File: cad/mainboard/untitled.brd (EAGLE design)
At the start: 100 x 80 mm, 12 parts

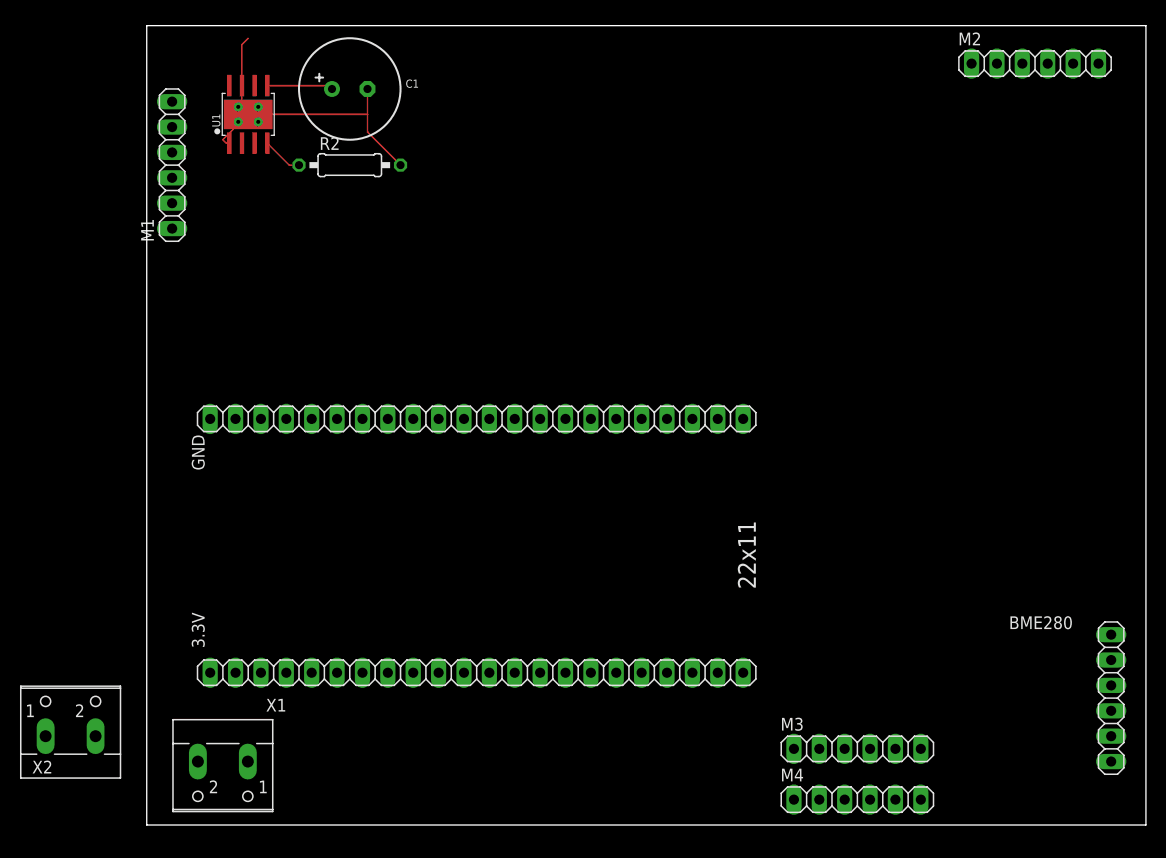
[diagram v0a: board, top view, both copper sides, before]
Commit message: board
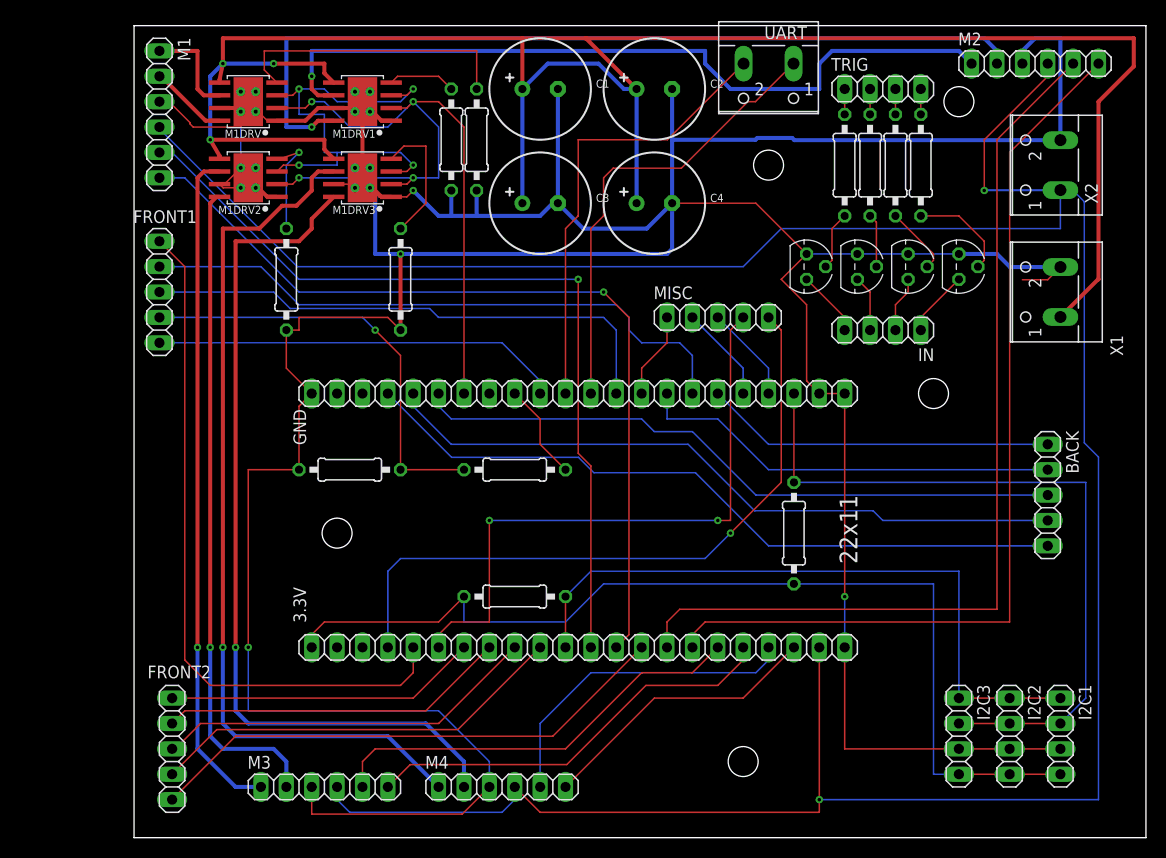
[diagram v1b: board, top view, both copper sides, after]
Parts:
- removed BME280: (no value), pinhead:1X06
- removed U1: (no value), Adafruit DRV8871:MICROBUILDER_HSOP8
- added 1K, 1K1, 1K3, 1K4, 1K5, 1K6, R3: 1k, rcl:0207/10
- added 1K2: 1.8k, rcl:0207/10
- added BACK, FRONT1, FRONT2, MISC: (no value), pinhead:1X05
- added C2, C3, C4: (no value), Adafruit DRV8871:MICROBUILDER_CELEC_3.5MM_10MM
- added I2C1, I2C2, I2C3, IN, TRIG: (no value), pinhead:1X04
- added M1DRV, M1DRV1, M1DRV2, M1DRV3: (no value), Adafruit DRV8871:MICROBUILDER_HSOP8
- added R1, R4, R5: 30k, rcl:0207/10
- added T1, T2, T3, T4: 2N3904, transistor:TO92
- added UART: (no value), con-wago-500:W237-102
- R2: value (none) -> 30k
- moved X2 112.6 mm to (90.2, 66.0), turned to 90 degrees
- moved X1 95.6 mm to (90.2, 53.3), turned to 90 degrees
- moved M3 53.5 mm to (17.8, 3.81)
- moved M4 35.6 mm to (35.6, 3.81)
- moved C1 19.0 mm to (39.4, 73.7)
- moved R2 13.0 mm to (33.0, 68.6), turned to 270 degrees
- moved 3.3V 10.5 mm to (43.2, 17.8)
- moved GND 10.5 mm to (43.2, 43.2)
- moved M1 5.24 mm to (1.27, 71.1), turned to 270 degrees
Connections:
- removed net M1S1: M1.5
- removed net M1S2: M1.6
- removed net M2S1: M2.5
- removed net M2S2: M2.6
- removed net M3S1: M3.5
- removed net M3S2: M3.6
- removed net M4S1: M4.5
- removed net M4S2: M4.6
- new net +3V3: 1K.1, 3.3V.1, I2C1.4, I2C2.4, I2C3.4, R3.1
- new net ARM2: BACK.1, GND.17
- new net IN: IN.1, T4.1
- new net N$1: M1DRV1.4, R1.1
- new net N$10: 1K3.2, TRIG.3
- new net N$11: IN.3, T2.1
- new net N$12: 1K4.1, T2.2
- new net N$13: 1K4.2, TRIG.2
- new net N$14: IN.4, T3.1
- new net N$15: 1K5.1, T3.2
- new net N$16: 1K5.2, TRIG.1
- new net N$18: 1K6.1, T4.2
- new net N$19: 1K6.2, TRIG.4
- new net N$2: M1DRV2.4, R4.1
- new net N$3: 1K1.1, GND.9
- new net N$4: M1DRV3.4, R5.1
- new net N$5: GND.11, UART.2
- new net N$6: GND.12, UART.1
- new net N$7: IN.2, T1.1
- new net N$8: 1K3.1, T1.2
- new net P0: GND.14, MISC.1
- new net P10: 3.3V.16, M2.6
- new net P11: 3.3V.17, M3.5
- new net P12: 3.3V.18, M3.6
- new net P13: 3.3V.19, M4.5
- new net P14: 3.3V.20, M4.6
- new net P15LASERX: 3.3V.8, FRONT2.4
- new net P16LASERY: 3.3V.9, FRONT2.3
- new net P17LASERTRIG: 3.3V.10, FRONT2.2
- new net P18SDA: 1K.2, 3.3V.11, I2C1.1, I2C2.1, I2C3.1
- new net P19SCL: GND.20, I2C1.2, I2C2.2, I2C3.2, R3.2
- new net P1ARM3: BACK.5, GND.4
- new net P20: GND.19, MISC.3
- new net P21: GND.18, MISC.2
- new net P2ARM4: BACK.4, GND.5
- new net P3: 3.3V.13, M1.6
- new net P35SONAR: FRONT1.3, GND.13
- new net P38SONARTRIG: FRONT1.5, GND.10
- new net P39SONARECHO: 1K1.2, 1K2.2, FRONT1.4
- new net P4: 3.3V.4, MISC.5
- new net P40: M1DRV.3, M1DRV1.3, M1DRV2.3, M1DRV3.3
- new net P40PWM2: GND.8
- new net P41PWM1: GND.7, M1DRV.2, M1DRV1.2, M1DRV2.2, M1DRV3.2
- new net P42ARM1: BACK.3, GND.6
- new net P43: GND.2
- new net P44: GND.3
- new net P45REARBUMP: BACK.2, GND.15
- new net P46FRONTBUMP: 3.3V.14, FRONT2.1
- new net P48LED: FRONT1.2, GND.16
- new net P5BUZZER: 3.3V.5, FRONT1.1
- new net P6: 3.3V.6, MISC.4
- new net P7STEER: 3.3V.7, FRONT2.5
- new net P8: 3.3V.12, M1.5
- new net P9: 3.3V.15, M2.5
- net +12V: now also C2.+, C3.+, C4.+, M1DRV.5, M1DRV1.5, M1DRV2.5, M1DRV3.5; no longer U1.5
- net +5V: now also 3.3V.21; no longer BME280.6
- net GND: now also 1K2.1, 3.3V.22, C2.-, C3.-, C4.-, GND.21, GND.22, I2C1.3, I2C2.3, I2C3.3, M1DRV.1, M1DRV.7, M1DRV.GND, M1DRV.P$1, M1DRV.P$2, M1DRV.P$3, M1DRV.P$4, M1DRV1.1, M1DRV1.7, M1DRV1.GND, M1DRV1.P$1, M1DRV1.P$2, M1DRV1.P$3, M1DRV1.P$4, M1DRV2.1, M1DRV2.7, M1DRV2.GND, M1DRV2.P$1, M1DRV2.P$2, M1DRV2.P$3, M1DRV2.P$4, M1DRV3.1, M1DRV3.7, M1DRV3.GND, M1DRV3.P$1, M1DRV3.P$2, M1DRV3.P$3, M1DRV3.P$4, R1.2, R4.2, R5.2, T1.3, T2.3, T3.3, T4.3; no longer BME280.5, U1.1, U1.7, U1.GND, U1.P$1, U1.P$2, U1.P$3, U1.P$4
- net M1+: now also M1DRV.6
- net M1-: now also M1DRV.8
- net M2+: now also M1DRV1.6
- net M2-: now also M1DRV1.8
- net M3+: now also M1DRV2.6
- net M3-: now also M1DRV2.8
- net M4+: now also M1DRV3.6
- net M4-: now also M1DRV3.8
- net N$9: now also M1DRV.4; no longer U1.4
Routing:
- net GND: track 32.6 -> 474.7 mm, vias 0 -> 4
- net +5V: track 0.00 -> 292.7 mm, vias 0 -> 2
- net +12V: track 6.62 -> 211.7 mm, vias 0 -> 3
- net +3V3: track 0.00 -> 100.9 mm
- net P9: track 0.00 -> 93.9 mm
- net P10: track 0.00 -> 93.1 mm
- net M4+: track 0.00 -> 88.0 mm, vias 0 -> 1
- net M2-: track 0.00 -> 86.8 mm, vias 0 -> 1
- net M4-: track 0.00 -> 86.7 mm, vias 0 -> 1
- net P3: track 0.00 -> 86.3 mm, vias 0 -> 1
- net P8: track 0.00 -> 84.5 mm, vias 0 -> 1
- net P41PWM1: track 0.00 -> 78.9 mm, vias 0 -> 4
- net M2+: track 0.00 -> 78.2 mm, vias 0 -> 1
- net P19SCL: track 0.00 -> 73.4 mm
- net P1ARM3: track 0.00 -> 72.4 mm
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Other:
- board size 100 x 80 mm -> 101.3 x 81.3 mm
- board text added: "+12"
- board text added: "1"
- board text added: "g"
- board text added: "p1"
- board text added: "p15"
- board text added: "p16"
- board text added: "p17"
- board text added: "p2"
- board text added: "p35"
- board text added: "p38"
- board text added: "p39"
- board text added: "p42"
- board text added: "p45"
- board text added: "p46"
- board text added: "p47"
- board text added: "p48"
- board text added: "p5"
- board text added: "p7"
